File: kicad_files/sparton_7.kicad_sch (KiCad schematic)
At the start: 0 parts

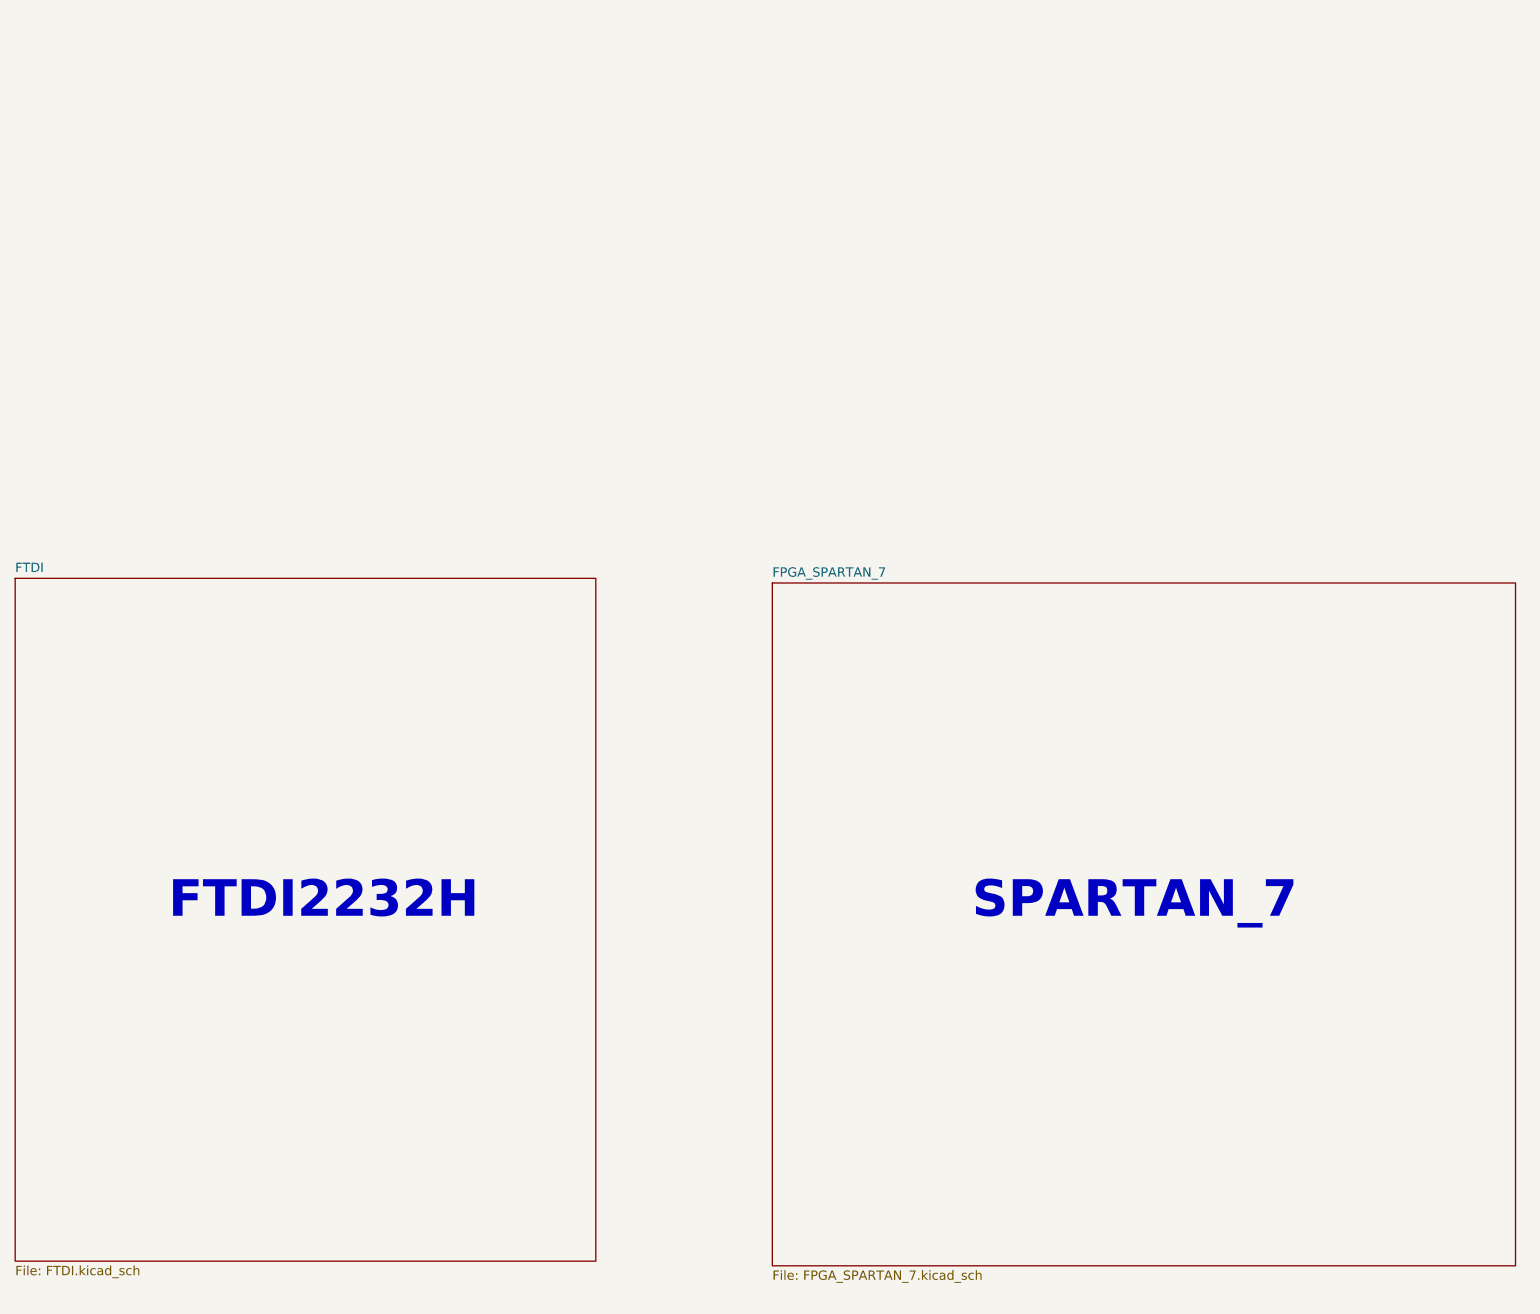
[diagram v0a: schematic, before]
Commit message: schematic updated
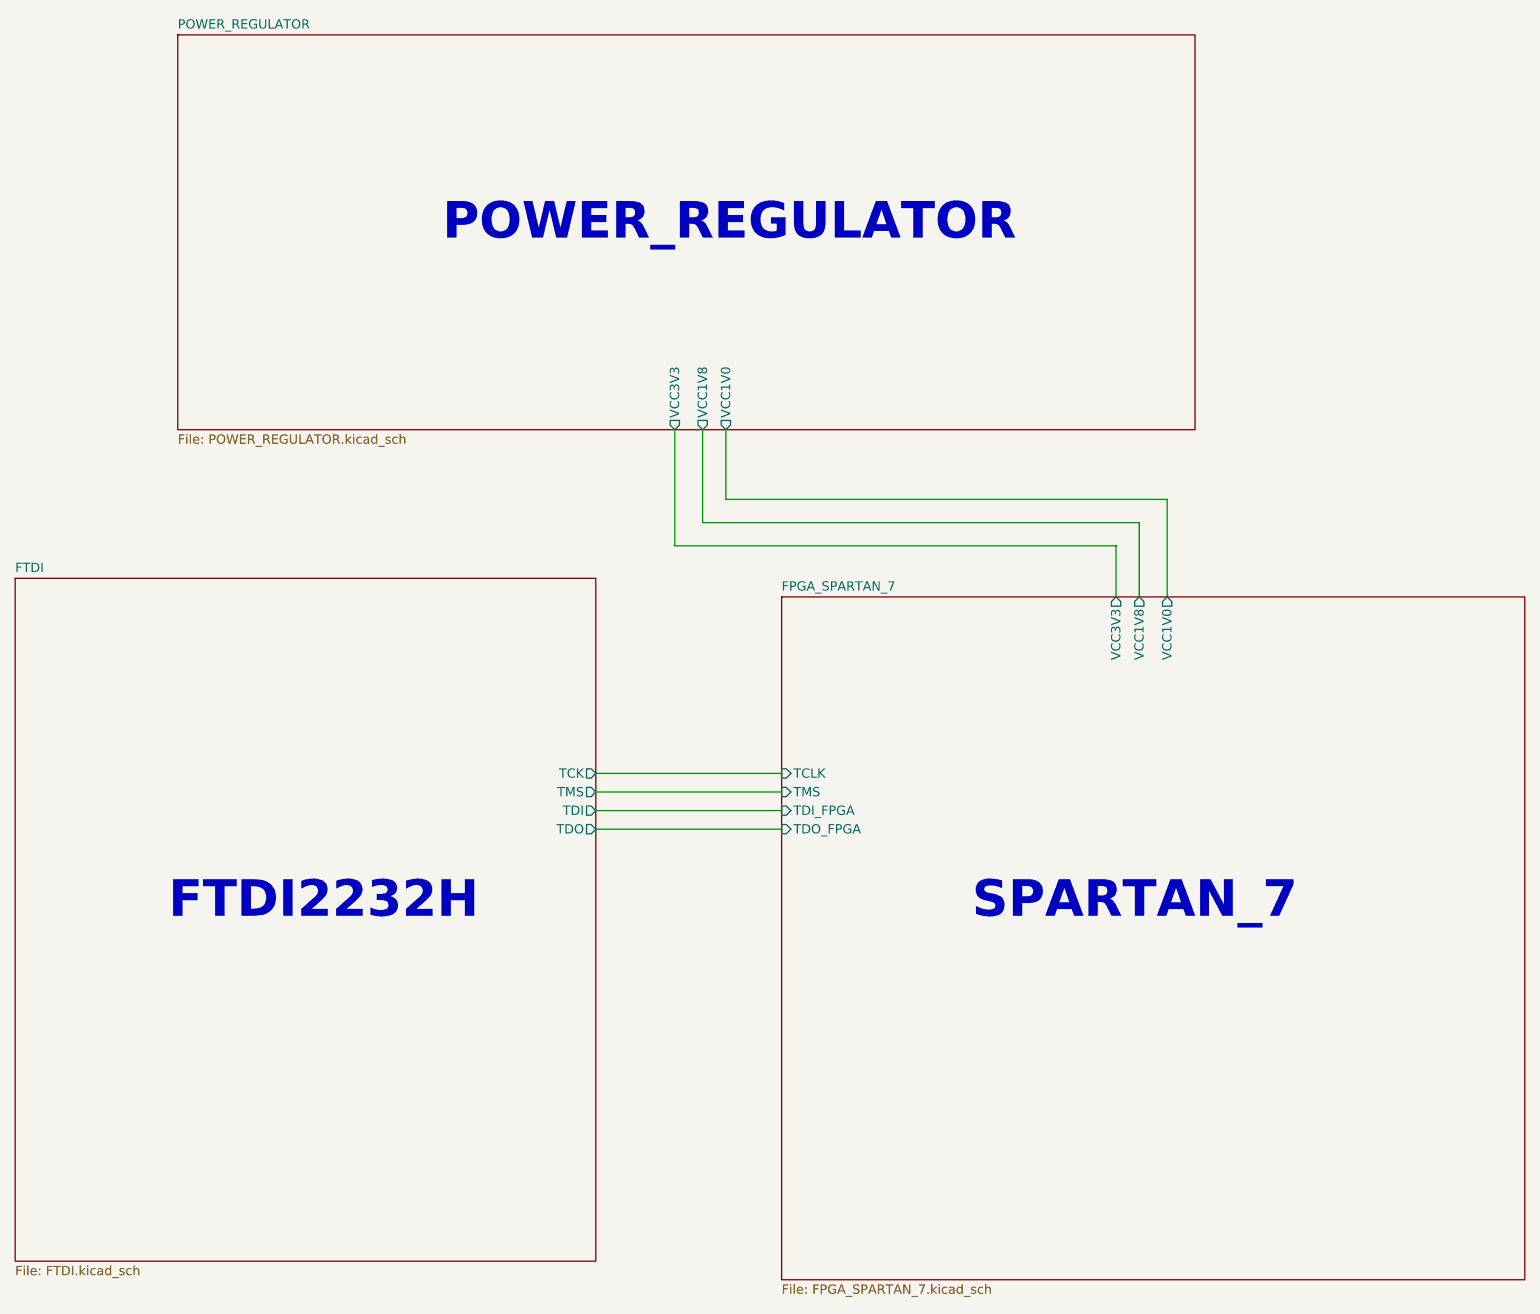
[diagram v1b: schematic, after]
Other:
- added sheet POWER_REGULATOR (POWER_REGULATOR.kicad_sch)
- sheet FPGA_SPARTAN_7 ports: added TCLK, TDI_FPGA, TDO_FPGA, TMS, VCC1V0, VCC1V8, VCC3V3; removed none
- sheet FTDI ports: added TCK, TDI, TDO, TMS; removed none
- note added: "POWER_REGULATOR"
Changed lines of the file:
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@@
 (kicad_sch (version 20230121) (generator eeschema)
   (paper "A3")
+  (wire (pts (xy 125.095 139.065) (xy 150.495 139.065))
+    (stroke (width 0) (type default))
+  )
+  (wire (pts (xy 139.7 102.235) (xy 199.39 102.235))
+    (stroke (width 0) (type default))
+  )
+  (wire (pts (xy 135.89 89.535) (xy 135.89 105.41))
+    (stroke (width 0) (type default))
+  )
+  (wire (pts (xy 139.7 89.535) (xy 139.7 102.235))
+    (stroke (width 0) (type default))
+  )
+  (wire (pts (xy 125.095 144.145) (xy 150.495 144.145))
+    (stroke (width 0) (type default))
+  )
+  (wire (pts (xy 135.89 105.41) (xy 196.215 105.41))
+    (stroke (width 0) (type default))
+  )
+  (wire (pts (xy 199.39 102.235) (xy 199.39 112.395))
+    (stroke (width 0) (type default))
+  )
+  (wire (pts (xy 142.875 99.06) (xy 203.2 99.06))
+    (stroke (width 0) (type default))
+  )
+  (wire (pts (xy 203.2 99.06) (xy 203.2 112.395))
+    (stroke (width 0) (type default))
+  )
+  (wire (pts (xy 196.215 105.41) (xy 196.215 112.395))
+    (stroke (width 0) (type default))
+  )
+  (wire (pts (xy 125.095 136.525) (xy 150.495 136.525))
+    (stroke (width 0) (type default))
+  )
+  (wire (pts (xy 125.095 141.605) (xy 150.495 141.605))
+    (stroke (width 0) (type default))
+  )
+  (wire (pts (xy 142.875 89.535) (xy 142.875 99.06))
+    (stroke (width 0) (type default))
+  )
   (text "FTDI2232H\n" (at 66.675 156.845 0)
     (effects (font (size 5 5) (thickness 0.6) bold) (justify left bottom))
@@
     (effects (font (size 5 5) (thickness 0.6) bold) (justify left bottom))
   )
-  (sheet (at 149.225 110.49) (size 101.6 93.345) (fields_autoplaced)
+  (text "POWER_REGULATOR\n" (at 104.14 64.135 0)
+    (effects (font (size 5 5) (thickness 0.6) bold) (justify left bottom))
+  )
+  (sheet (at 67.945 35.56) (size 139.065 53.975) (fields_autoplaced)
     (stroke (width 0.1524) (type solid))
     (fill (color 0 0 0 0.0000))
-    (property "Sheetname" "FPGA_SPARTAN_7" (at 149.225 109.7784 0)
+    (property "Sheetname" "POWER_REGULATOR" (at 67.945 34.8484 0)
       (effects (font (size 1.27 1.27)) (justify left bottom))
     )
-    (property "Sheetfile" "FPGA_SPARTAN_7.kicad_sch" (at 149.225 204.4196 0)
+    (property "Sheetfile" "POWER_REGULATOR.kicad_sch" (at 67.945 90.1196 0)
       (effects (font (size 1.27 1.27)) (justify left top))
+    )
+    (property "Field2" "" (at 67.945 35.56 0)
+      (effects (font (size 1.27 1.27)) hide)
+    )
+    (pin "VCC1V0" output (at 142.875 89.535 270)
+      (effects (font (size 1.27 1.27)) (justify left))
+    )
+    (pin "VCC1V8" output (at 139.7 89.535 270)
+      (effects (font (size 1.27 1.27)) (justify left))
+    )
+    (pin "VCC3V3" output (at 135.89 89.535 270)
+      (effects (font (size 1.27 1.27)) (justify left))
+    )
+    (instances
+      (project "sparton_7"
+        (path "/94bd3a84-5526-4cf2-a5cc-3887356f447c" (page "9"))
+      )
+    )
+  )
+  (sheet (at 150.495 112.395) (size 101.6 93.345) (fields_autoplaced)
+    (stroke (width 0.1524) (type solid))
+    (fill (color 0 0 0 0.0000))
+    (property "Sheetname" "FPGA_SPARTAN_7" (at 150.495 111.6834 0)
+      (effects (font (size 1.27 1.27)) (justify left bottom))
+    )
+    (property "Sheetfile" "FPGA_SPARTAN_7.kicad_sch" (at 150.495 206.3246 0)
+      (effects (font (size 1.27 1.27)) (justify left top))
+    )
+    (pin "TDI_FPGA" input (at 150.495 141.605 180)
+      (effects (font (size 1.27 1.27)) (justify left))
+    )
+    (pin "TMS" input (at 150.495 139.065 180)
+      (effects (font (size 1.27 1.27)) (justify left))
+    )
+    (pin "TCLK" input (at 150.495 136.525 180)
+      (effects (font (size 1.27 1.27)) (justify left))
+    )
+    (pin "TDO_FPGA" input (at 150.495 144.145 180)
+      (effects (font (size 1.27 1.27)) (justify left))
+    )
+    (pin "VCC1V8" output (at 199.39 112.395 90)
+      (effects (font (size 1.27 1.27)) (justify right))
+    )
+    (pin "VCC1V0" output (at 203.2 112.395 90)
+      (effects (font (size 1.27 1.27)) (justify right))
+    )
+    (pin "VCC3V3" output (at 196.215 112.395 90)
+      (effects (font (size 1.27 1.27)) (justify right))
     )
     (instances
@@
       (effects (font (size 1.27 1.27)) hide)
     )
+    (pin "TMS" output (at 125.095 139.065 0)
+      (effects (font (size 1.27 1.27)) (justify right))
+    )
+    (pin "TDO" output (at 125.095 144.145 0)
+      (effects (font (size 1.27 1.27)) (justify right))
+    )
+    (pin "TDI" output (at 125.095 141.605 0)
+      (effects (font (size 1.27 1.27)) (justify right))
+    )
+    (pin "TCK" output (at 125.095 136.525 0)
+      (effects (font (size 1.27 1.27)) (justify right))
+    )
     (instances
